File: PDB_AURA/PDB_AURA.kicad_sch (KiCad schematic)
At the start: 0 parts

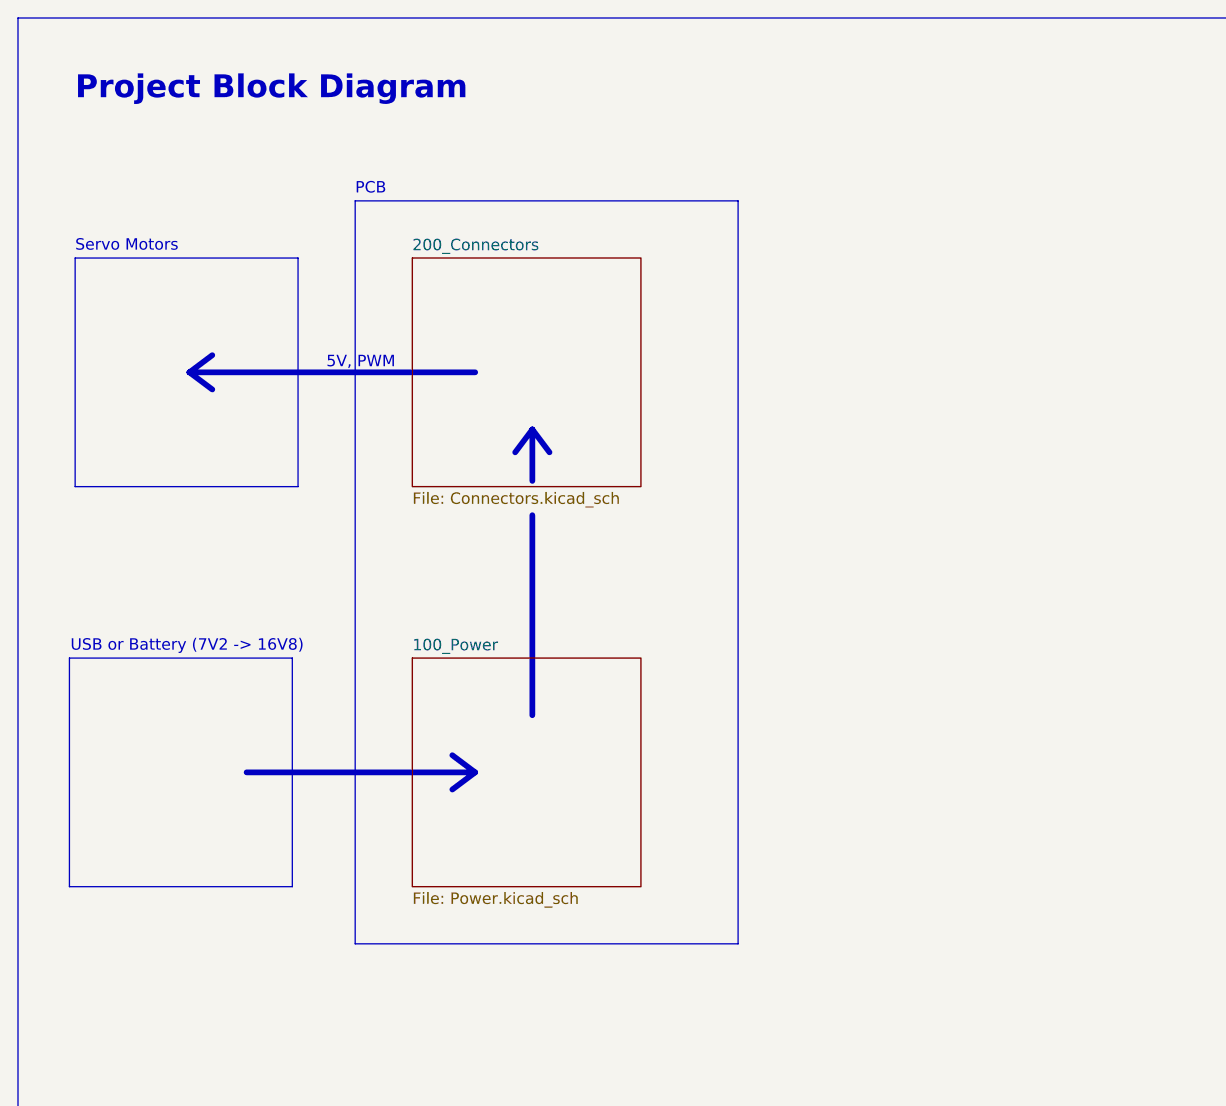
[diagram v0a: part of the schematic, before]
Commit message: Moving to laptop
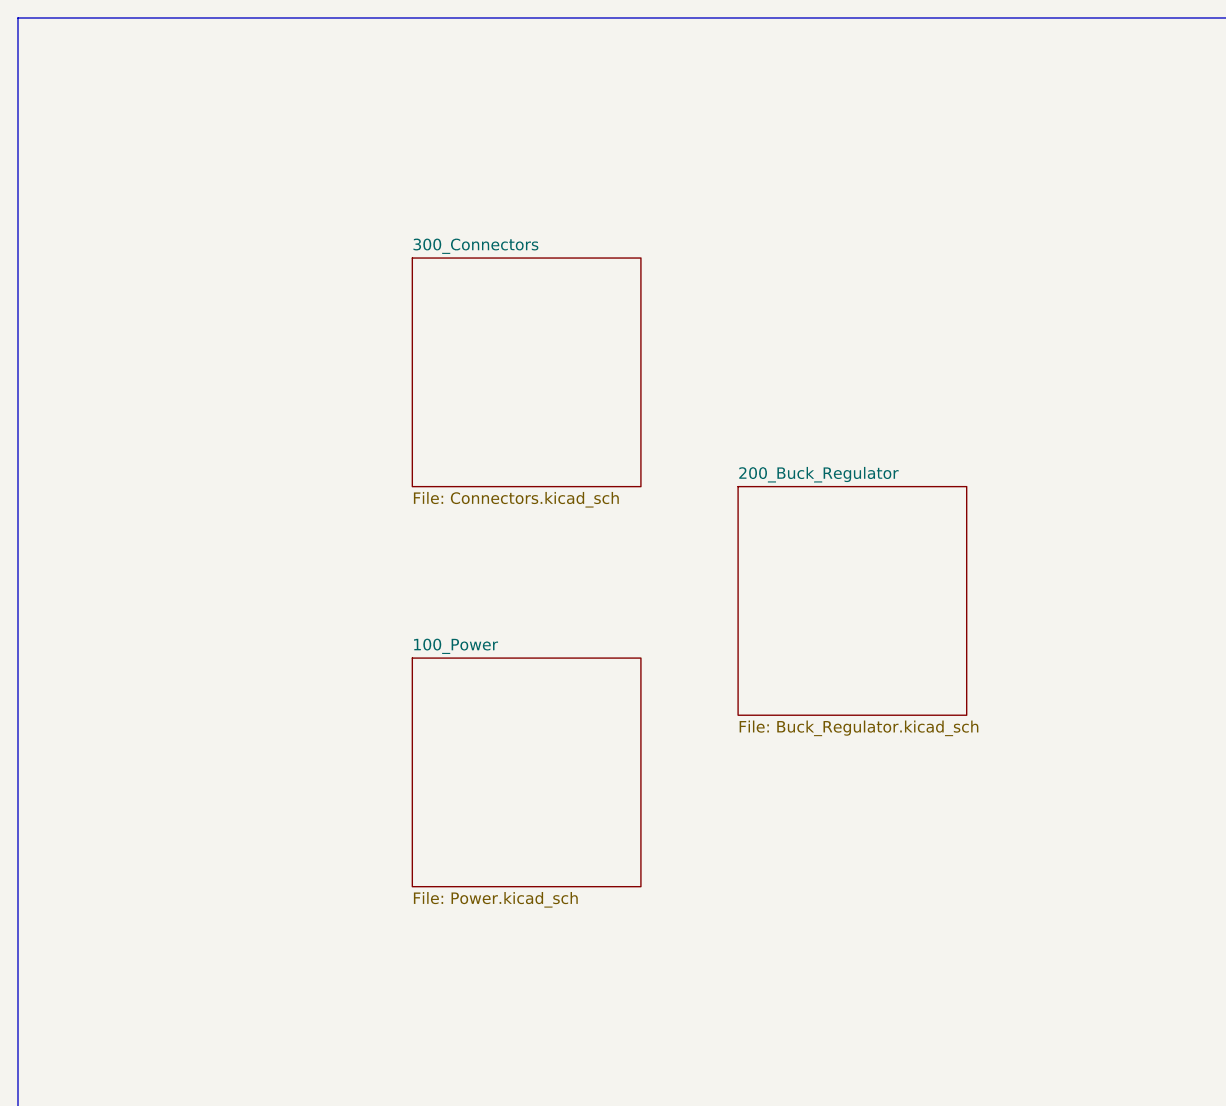
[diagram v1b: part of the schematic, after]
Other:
- sheet 200_Connectors renamed 300_Connectors
- added sheet 200_Buck_Regulator (Buck_Regulator.kicad_sch)
- note removed: "5V, PWM"
- note removed: "PCB"
- note removed: "Project Block Diagram"
- note removed: "Servo Motors"
- note removed: "USB or Battery (7V2 -> 16V8)"
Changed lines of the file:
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@@
-		)
-	)
-	(rectangle
-		(start 27.305 95.25)
-		(end 52.07 120.65)
-		(stroke
-			(width 0)
-			(type solid)
-		)
-		(fill
-			(type none)
-		)
-	)
-	(rectangle
-		(start 59.055 44.45)
-		(end 101.6 127)
-		(stroke
-			(width 0)
-			(type default)
-		)
-		(fill
-			(type none)
-		)
-	)
-	(rectangle
-		(start 27.94 50.8)
-		(end 52.705 76.2)
-		(stroke
-			(width 0)
-			(type solid)
-		)
-		(fill
-			(type none)
 		)
 	)
@@
 		)
 	)
-	(text "PCB"
-		(exclude_from_sim no)
-		(at 59.055 43.18 0)
-		(effects
-			(font
-				(size 1.27 1.27)
-			)
-			(justify left)
-		)
-	)
-	(text "5V, PWM"
-		(exclude_from_sim no)
-		(at 59.69 62.484 0)
-		(effects
-			(font
-				(size 1.27 1.27)
-			)
-		)
-	)
 	(text "Maybe switch regulator to SiC437/SiC431.\n\nConfirm power specifications.\n\nFix block diagram (it is outdated)."
 		(exclude_from_sim no)
@@
 			)
 			(justify left top)
-		)
-	)
-	(text "Project Block Diagram\n"
-		(exclude_from_sim no)
-		(at 27.94 32.004 0)
-		(effects
-			(font
-				(size 2.54 2.54)
-				(thickness 0.508)
-				(bold yes)
-			)
-			(justify left)
-		)
-	)
-	(text "USB or Battery (7V2 -> 16V8)\n"
-		(exclude_from_sim no)
-		(at 40.386 93.98 0)
-		(effects
-			(font
-				(size 1.27 1.27)
-			)
 		)
 	)
@@
 			)
 			(justify left)
-		)
-	)
-	(text "Servo Motors"
-		(exclude_from_sim no)
-		(at 27.94 49.53 0)
-		(effects
-			(font
-				(size 1.27 1.27)
-			)
-			(justify left)
-		)
-	)
-	(polyline
-		(pts
-			(xy 40.64 63.5) (xy 43.18 61.595)
-		)
-		(stroke
-			(width 0.635)
-			(type solid)
-		)
-	)
-	(polyline
-		(pts
-			(xy 78.74 69.85) (xy 76.835 72.39)
-		)
-		(stroke
-			(width 0.635)
-			(type solid)
-		)
-	)
-	(polyline
-		(pts
-			(xy 72.39 107.95) (xy 69.85 109.855)
-		)
-		(stroke
-			(width 0.635)
-			(type solid)
-		)
-	)
-	(polyline
-		(pts
-			(xy 78.74 79.375) (xy 78.74 101.6)
-		)
-		(stroke
-			(width 0.635)
-			(type solid)
-		)
-	)
-	(polyline
-		(pts
-			(xy 46.99 107.95) (xy 71.755 107.95)
-		)
-		(stroke
-			(width 0.635)
-			(type solid)
-		)
-	)
-	(polyline
-		(pts
-			(xy 40.64 63.5) (xy 72.39 63.5)
-		)
-		(stroke
-			(width 0.635)
-			(type solid)
-		)
-	)
-	(polyline
-		(pts
-			(xy 40.64 63.5) (xy 43.18 65.405)
-		)
-		(stroke
-			(width 0.635)
-			(type solid)
-		)
-	)
-	(polyline
-		(pts
-			(xy 78.74 69.85) (xy 78.74 75.565)
-		)
-		(stroke
-			(width 0.635)
-			(type solid)
-		)
-	)
-	(polyline
-		(pts
-			(xy 72.39 107.95) (xy 69.85 106.045)
-		)
-		(stroke
-			(width 0.635)
-			(type solid)
-		)
-	)
-	(polyline
-		(pts
-			(xy 78.74 69.85) (xy 80.645 72.39)
-		)
-		(stroke
-			(width 0.635)
-			(type solid)
 		)
 	)
@@
 			(color 0 0 0 0.0000)
 		)
-		(property "Sheetname" "200_Connectors"
+		(property "Sheetname" "300_Connectors"
 			(at 65.405 50.0884 0)
 			(effects
@@
 			(project "PDB_AURA"
 				(path "/c0b09de1-c640-438f-9ef5-dda14a6aac71"
-					(page "3")
+					(page "4")
 				)
 			)
@@
 				)
 			)
+		)
+	)
+	(sheet
+		(at 101.6 76.2)
+		(size 25.4 25.4)
+		(exclude_from_sim no)
+		(in_bom yes)
+		(on_board yes)
+		(dnp no)
+		(fields_autoplaced yes)
+		(stroke
+			(width 0.1524)
+			(type solid)
+		)
+		(fill
+			(color 0 0 0 0.0000)
+		)
+		(property "Sheetname" "200_Buck_Regulator"
+			(at 101.6 75.4884 0)
+			(effects
+				(font
+					(size 1.27 1.27)
+				)
+				(justify left bottom)
+			)
+		)
+		(property "Sheetfile" "Buck_Regulator.kicad_sch"
+			(at 101.6 102.1846 0)
+			(effects
+				(font
+					(size 1.27 1.27)
+				)
+				(justify left top)
+			)
+		)
+		(instances
+			(project "PDB_AURA"
+				(path "/c0b09de1-c640-438f-9ef5-dda14a6aac71"
+					(page "3")
+				)
+			)
